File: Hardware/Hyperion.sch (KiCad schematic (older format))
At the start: 2 parts

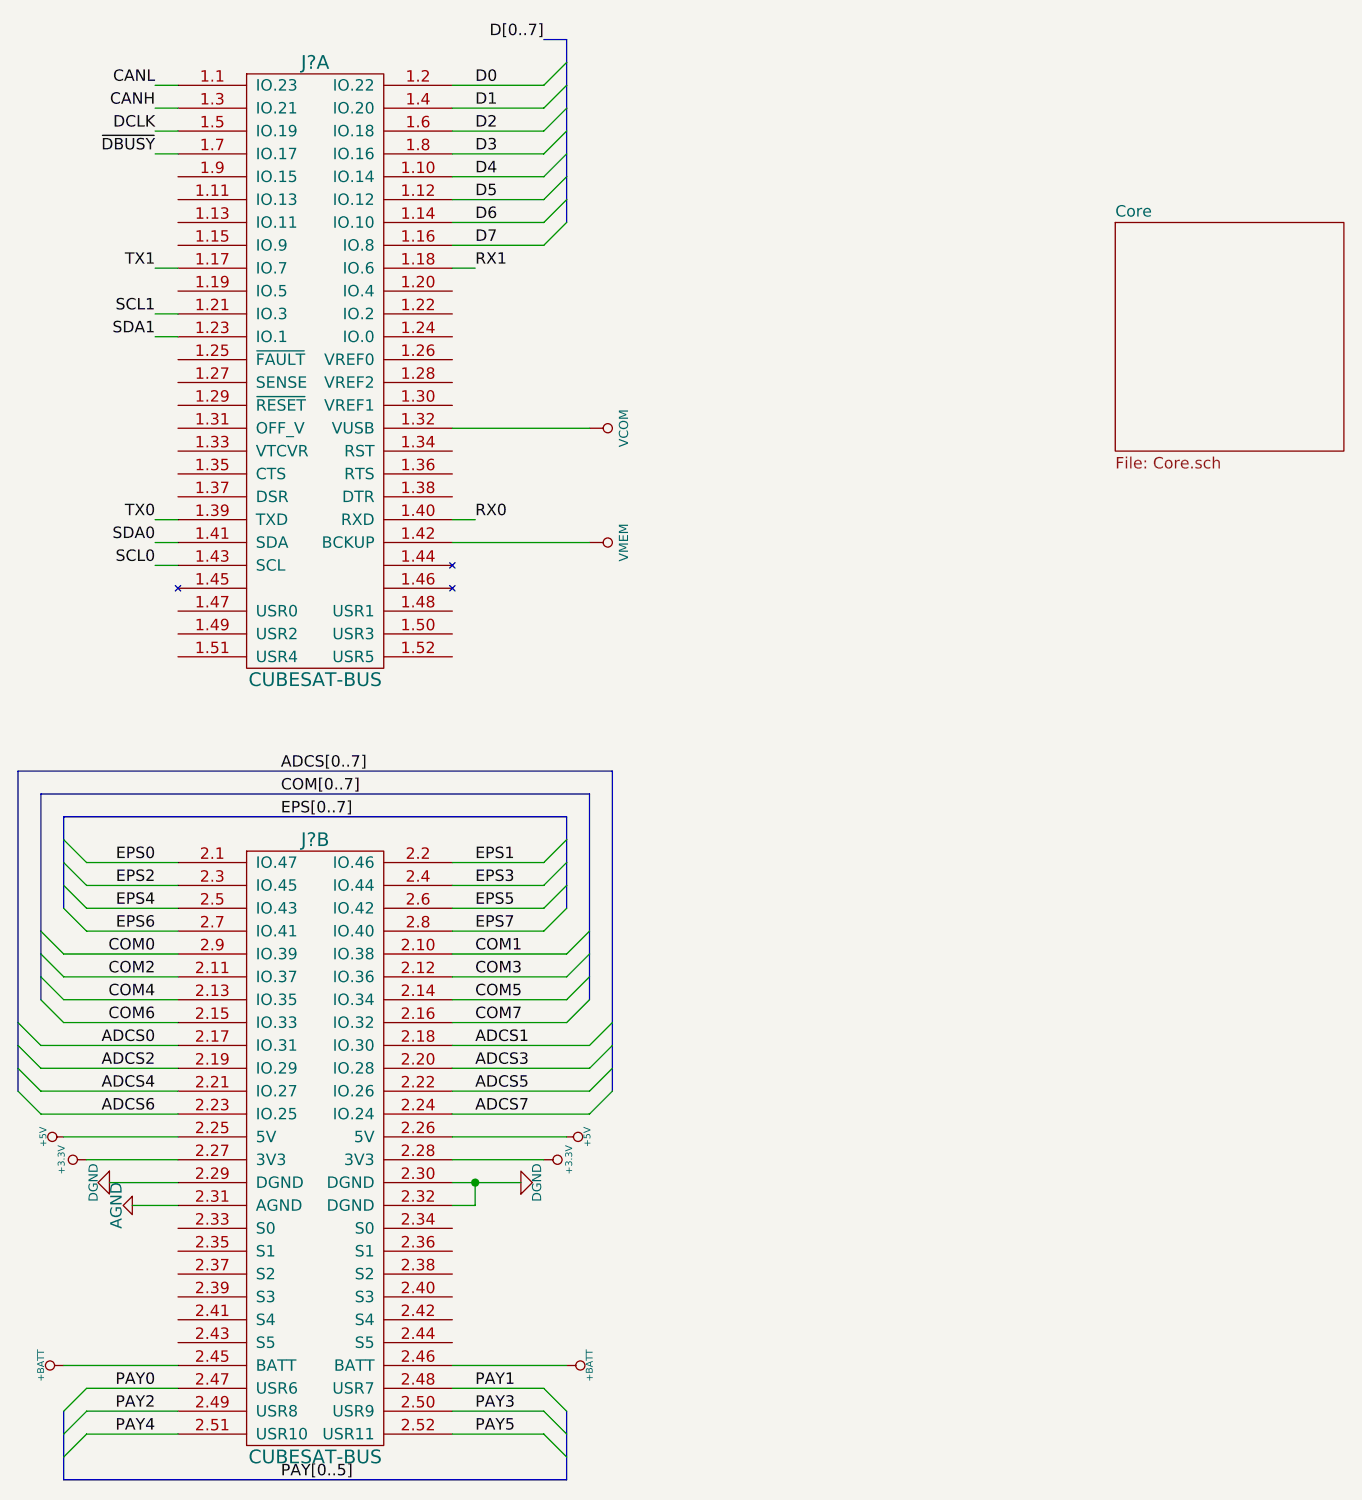
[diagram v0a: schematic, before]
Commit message: Save annotation
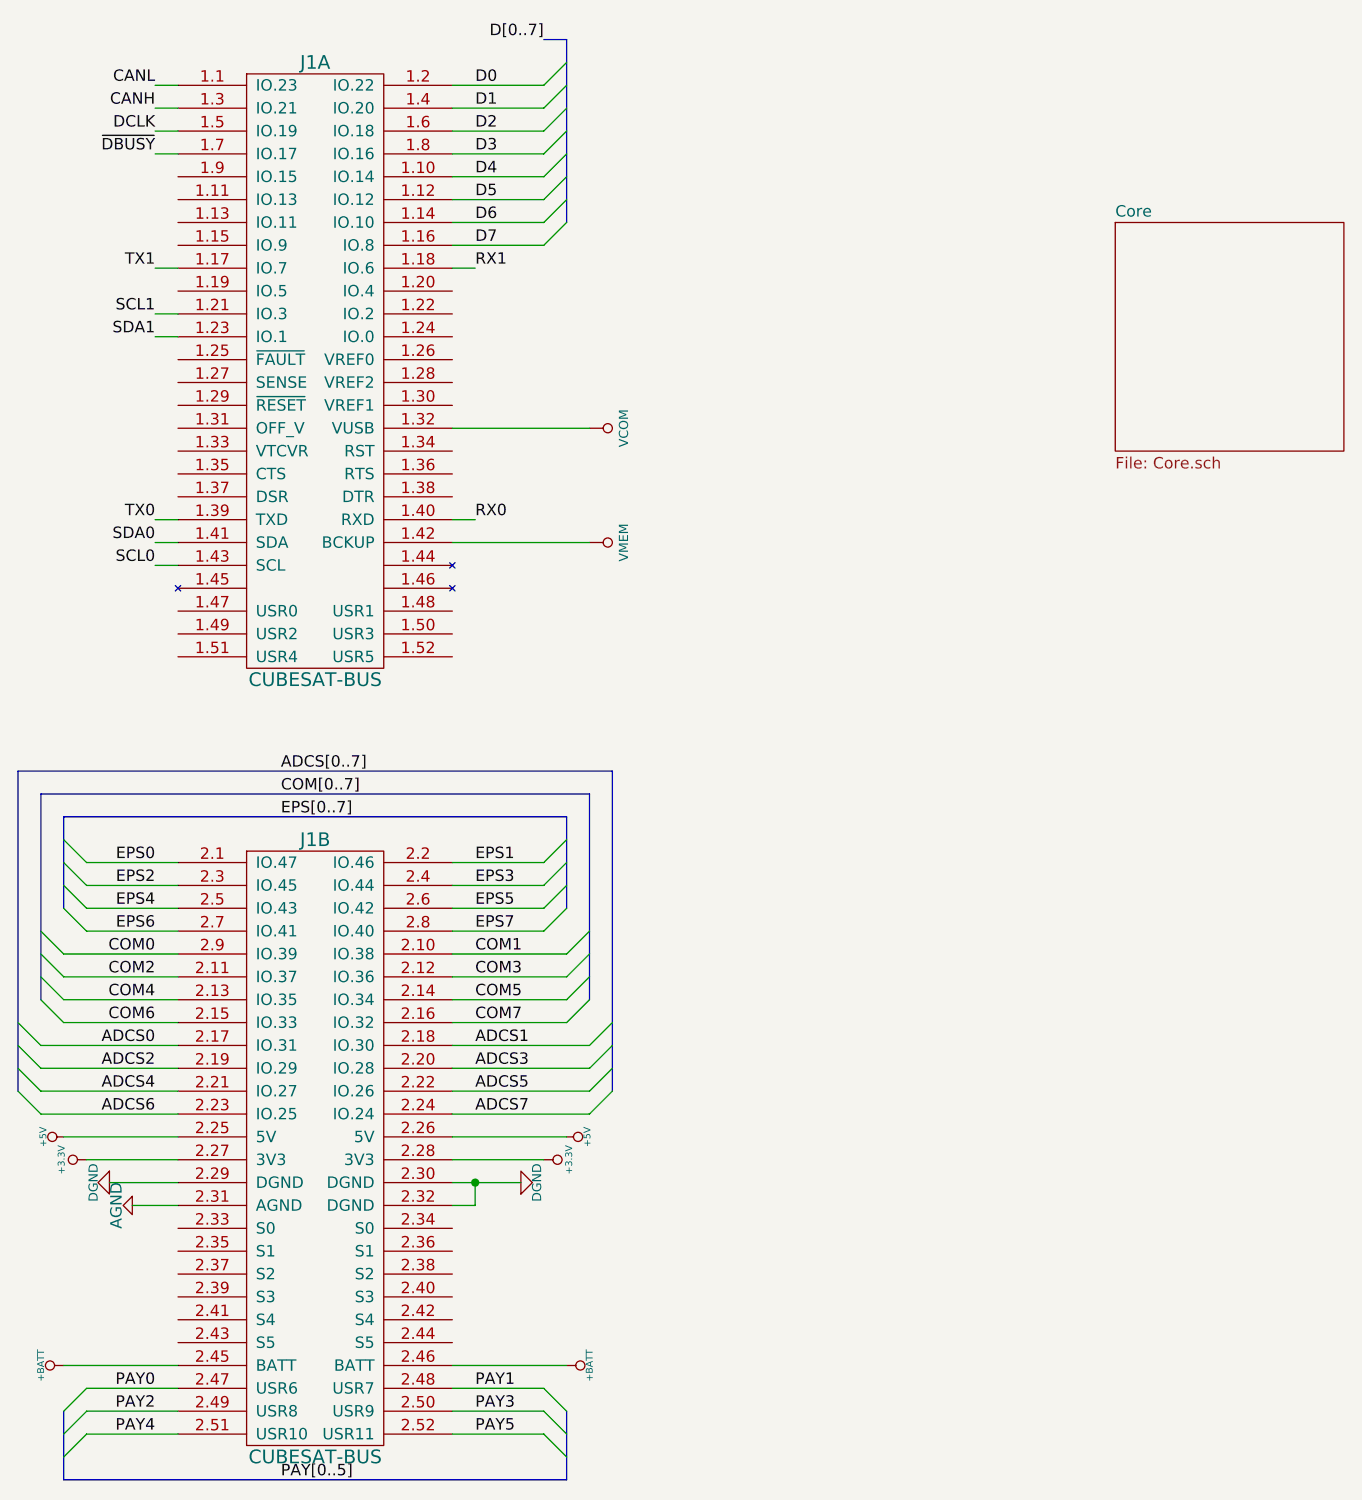
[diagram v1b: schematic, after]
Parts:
- gave numbers to parts that had none: 1
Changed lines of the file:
@@
 $EndDescr
 $Comp
-L CUBESAT-BUS J?
+L CUBESAT-BUS J1
 U 1 1 5253906A
 P 2000 2350
-F 0 "J?" H 2000 3700 60  0000 C CNN
+F 0 "J1" H 2000 3700 60  0000 C CNN
 F 1 "CUBESAT-BUS" H 2000 1000 60  0000 C CNN
 F 2 "" H 2000 2350 60  0000 C CNN
@@
 $EndComp
 $Comp
-L CUBESAT-BUS J?
+L CUBESAT-BUS J1
 U 2 1 52539079
 P 2000 5750
-F 0 "J?" H 2000 7100 60  0000 C CNN
+F 0 "J1" H 2000 7100 60  0000 C CNN
 F 1 "CUBESAT-BUS" H 2000 4400 60  0000 C CNN
 F 2 "" H 2000 5750 60  0000 C CNN
@@
 D7
 $Comp
-L VMEM #PWR?
+L VMEM #PWR11
 U 1 1 52FF2E7C
 P 3200 3100
-F 0 "#PWR?" H 3200 3300 40  0001 C CNN
+F 0 "#PWR11" H 3200 3300 40  0001 C CNN
 F 1 "VMEM" H 3200 3250 40  0000 C CNN
 F 2 "" H 3200 3100 60  0000 C CNN
@@
 $EndComp
 $Comp
-L VCOM #PWR?
+L VCOM #PWR10
 U 1 1 52FF2EBE
 P 3200 2600
-F 0 "#PWR?" H 3200 2800 40  0001 C CNN
+F 0 "#PWR10" H 3200 2800 40  0001 C CNN
 F 1 "VCOM" H 3200 2750 40  0000 C CNN
 F 2 "" H 3200 2600 60  0000 C CNN
@@
 $EndComp
 $Comp
-L +5V #PWR?
+L +5V #PWR8
 U 1 1 52FF2F36
 P 3100 5700
-F 0 "#PWR?" H 3100 5790 20  0001 C CNN
+F 0 "#PWR8" H 3100 5790 20  0001 C CNN
 F 1 "+5V" H 3100 5790 30  0000 C CNN
 F 2 "" H 3100 5700 60  0000 C CNN
@@
 $EndComp
 $Comp
-L +5V #PWR?
+L +5V #PWR1
 U 1 1 52FF2F45
 P 900 5700
-F 0 "#PWR?" H 900 5790 20  0001 C CNN
+F 0 "#PWR1" H 900 5790 20  0001 C CNN
 F 1 "+5V" H 900 5790 30  0000 C CNN
 F 2 "" H 900 5700 60  0000 C CNN
@@
 $EndComp
 $Comp
-L +3.3V #PWR?
+L +3.3V #PWR3
 U 1 1 52FF2F54
 P 1000 5800
-F 0 "#PWR?" H 1000 5760 30  0001 C CNN
+F 0 "#PWR3" H 1000 5760 30  0001 C CNN
 F 1 "+3.3V" H 1000 5910 30  0000 C CNN
 F 2 "" H 1000 5800 60  0000 C CNN
@@
 $EndComp
 $Comp
-L +3.3V #PWR?
+L +3.3V #PWR7
 U 1 1 52FF2F63
 P 3000 5800
-F 0 "#PWR?" H 3000 5760 30  0001 C CNN
+F 0 "#PWR7" H 3000 5760 30  0001 C CNN
 F 1 "+3.3V" H 3000 5910 30  0000 C CNN
 F 2 "" H 3000 5800 60  0000 C CNN
@@
 $EndComp
 $Comp
-L DGND #PWR?
+L DGND #PWR4
 U 1 1 52FF2F72
 P 1100 5900
-F 0 "#PWR?" H 1100 5900 40  0001 C CNN
+F 0 "#PWR4" H 1100 5900 40  0001 C CNN
 F 1 "DGND" H 1100 5830 40  0000 C CNN
 F 2 "" H 1100 5900 60  0000 C CNN
@@
 $EndComp
 $Comp
-L DGND #PWR?
+L DGND #PWR6
 U 1 1 52FF2F81
 P 2900 5900
-F 0 "#PWR?" H 2900 5900 40  0001 C CNN
+F 0 "#PWR6" H 2900 5900 40  0001 C CNN
 F 1 "DGND" H 2900 5830 40  0000 C CNN
 F 2 "" H 2900 5900 60  0000 C CNN
@@
 $EndComp
 $Comp
-L +BATT #PWR?
+L +BATT #PWR9
 U 1 1 52FF2F9F
 P 3100 6700
-F 0 "#PWR?" H 3100 6650 20  0001 C CNN
+F 0 "#PWR9" H 3100 6650 20  0001 C CNN
 F 1 "+BATT" H 3100 6800 30  0000 C CNN
 F 2 "" H 3100 6700 60  0000 C CNN
@@
 $EndComp
 $Comp
-L +BATT #PWR?
+L +BATT #PWR2
 U 1 1 52FF2FAE
 P 900 6700
-F 0 "#PWR?" H 900 6650 20  0001 C CNN
+F 0 "#PWR2" H 900 6650 20  0001 C CNN
 F 1 "+BATT" H 900 6800 30  0000 C CNN
 F 2 "" H 900 6700 60  0000 C CNN
@@
 $EndComp
 $Comp
-L AGND #PWR?
+L AGND #PWR5
 U 1 1 52FF3031
 P 1200 6000
-F 0 "#PWR?" H 1200 6000 40  0001 C CNN
+F 0 "#PWR5" H 1200 6000 40  0001 C CNN
 F 1 "AGND" H 1200 5930 50  0000 C CNN
 F 2 "" H 1200 6000 60  0000 C CNN
@@
 	2600 5800 3000 5800
 Wire Wire Line
-	2600 5900 2700 5900
-Wire Wire Line
-	2700 5900 2900 5900
+	2600 5900 2900 5900
 Wire Wire Line
 	3100 6700 2600 6700
@@
 	1400 6700 900  6700
 Wire Bus Line
-	900  4300 900  4400
-Wire Bus Line
-	900  4400 900  4500
-Wire Bus Line
-	900  4500 900  4600
-Wire Bus Line
-	900  4600 900  4700
+	900  4300 900  4700
 Wire Bus Line
 	900  4300 3100 4300
 Wire Bus Line
-	3100 4300 3100 4400
-Wire Bus Line
-	3100 4400 3100 4500
-Wire Bus Line
-	3100 4500 3100 4600
-Wire Bus Line
-	3100 4600 3100 4700
-Wire Bus Line
-	800  4200 800  4800
-Wire Bus Line
-	800  4800 800  4900
-Wire Bus Line
-	800  4900 800  5000
-Wire Bus Line
-	800  5000 800  5100
+	3100 4300 3100 4700
+Wire Bus Line
+	800  4200 800  5100
 Wire Bus Line
 	800  4200 3200 4200
 Wire Bus Line
-	3200 4200 3200 4800
-Wire Bus Line
-	3200 4800 3200 4900
-Wire Bus Line
-	3200 4900 3200 5000
-Wire Bus Line
-	3200 5000 3200 5100
-Wire Bus Line
-	700  4100 700  5200
-Wire Bus Line
-	700  5200 700  5300
-Wire Bus Line
-	700  5300 700  5400
-Wire Bus Line
-	700  5400 700  5500
+	3200 4200 3200 5100
+Wire Bus Line
+	700  4100 700  5500
 Wire Bus Line
 	700  4100 3300 4100
 Wire Bus Line
-	3300 4100 3300 5200
-Wire Bus Line
-	3300 5200 3300 5300
-Wire Bus Line
-	3300 5300 3300 5400
-Wire Bus Line
-	3300 5400 3300 5500
-Wire Bus Line
-	900  6900 900  7000
-Wire Bus Line
-	900  7000 900  7100
-Wire Bus Line
-	900  7100 900  7200
-Wire Bus Line
-	3100 7200 3100 7100
-Wire Bus Line
-	3100 7100 3100 7000
-Wire Bus Line
-	3100 7000 3100 6900
+	3300 4100 3300 5500
+Wire Bus Line
+	900  6900 900  7200
+Wire Bus Line
+	3100 6900 3100 7200
 Wire Wire Line
 	2600 6000 2700 6000
@@
 Connection ~ 2700 5900
 Wire Bus Line
-	900  7200 3100 7200
+	3100 7200 900  7200
 Entry Wire Line
 	3000 1100 3100 1000
@@
 	3000 1800 3100 1700
 Wire Bus Line
-	3100 1700 3100 1600
-Wire Bus Line
-	3100 1600 3100 1500
-Wire Bus Line
-	3100 1500 3100 1400
-Wire Bus Line
-	3100 1400 3100 1300
-Wire Bus Line
-	3100 1300 3100 1200
-Wire Bus Line
-	3100 1200 3100 1100
-Wire Bus Line
-	3100 1100 3100 1000
-Wire Bus Line
-	3100 1000 3100 900
+	3100 900  3100 1700
 Wire Bus Line
 	3100 900  3000 900
